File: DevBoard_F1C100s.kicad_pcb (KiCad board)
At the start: 2 copper layers, 192.8 x 140.2 mm, 51 parts, among them J101 USB_C_Receptacle_USB2.0_16P, J102 Conn_01x22, J103 Conn_01x11, J104 SD_Card, J105 UART0, J106 Conn_01x10, J108 Conn_01x05, J109 Conn_01x02, SW101 SW0, SW102 SW1, SW103 SW2, SW104 SW3, SW105 RESET, U101 AMS1117, U102 AMS1117-3.3, U103 TPS562201DDCT, U104 W25Q16JVSS, U105 F1C100s, Y101 24Mhz

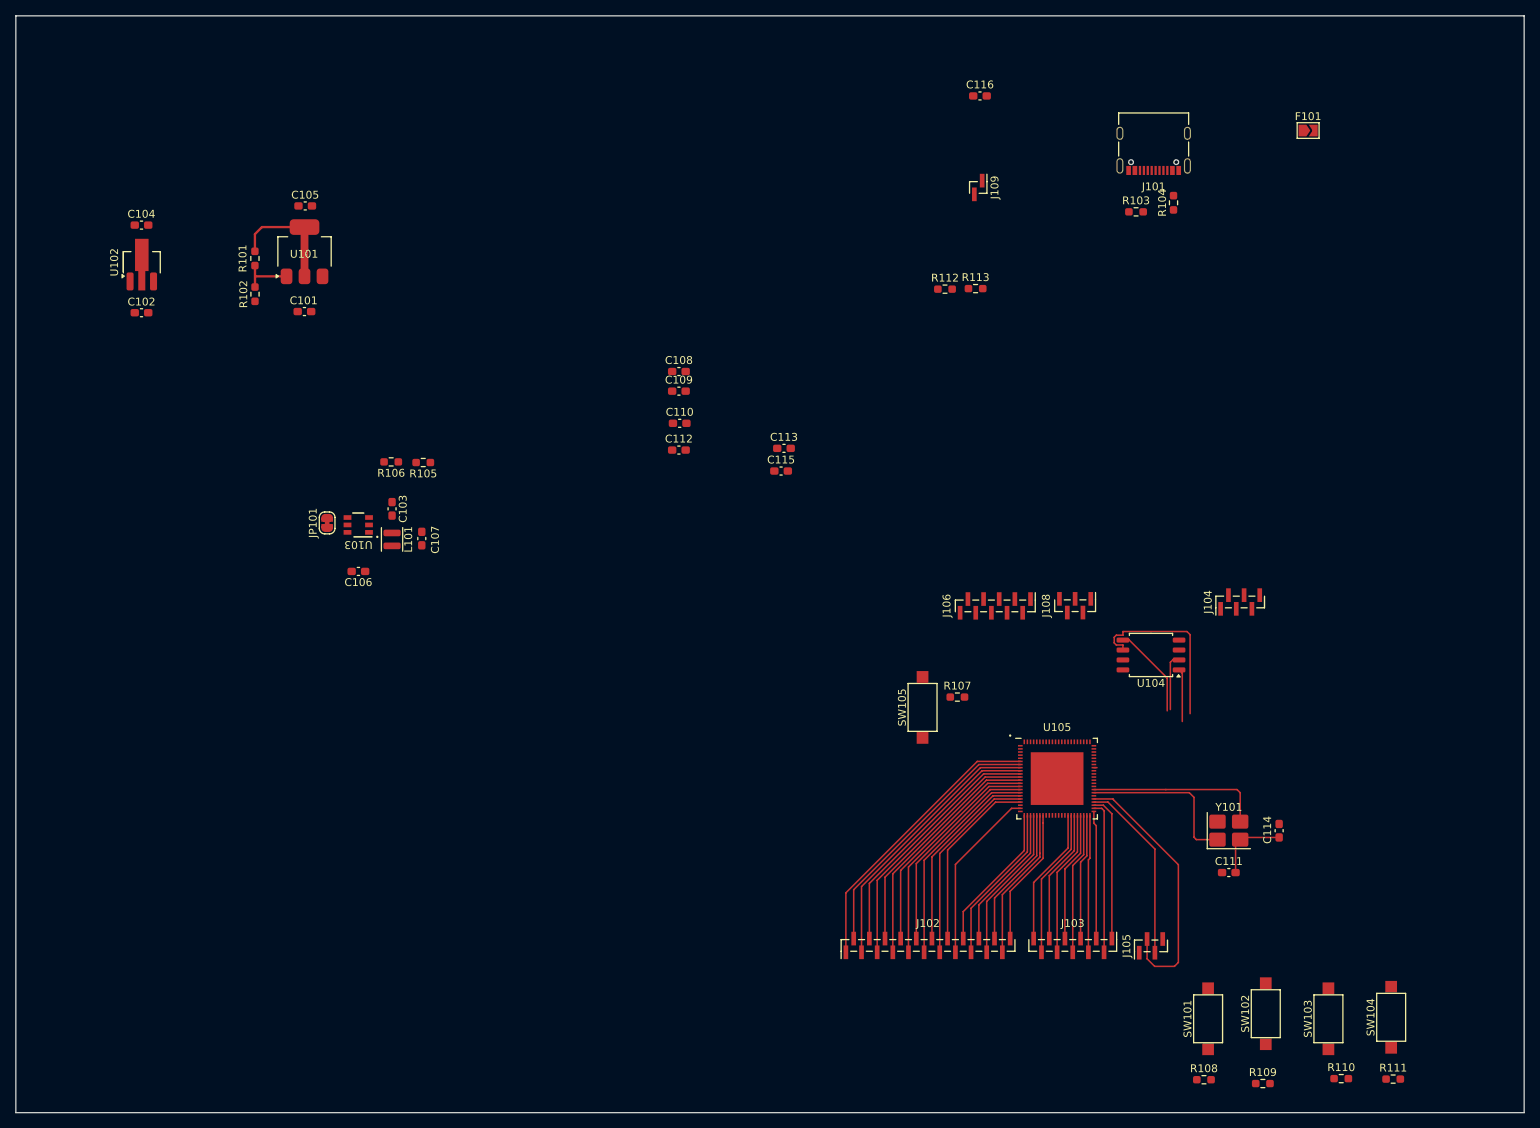
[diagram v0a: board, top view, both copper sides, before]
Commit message: Layout: Almost complete
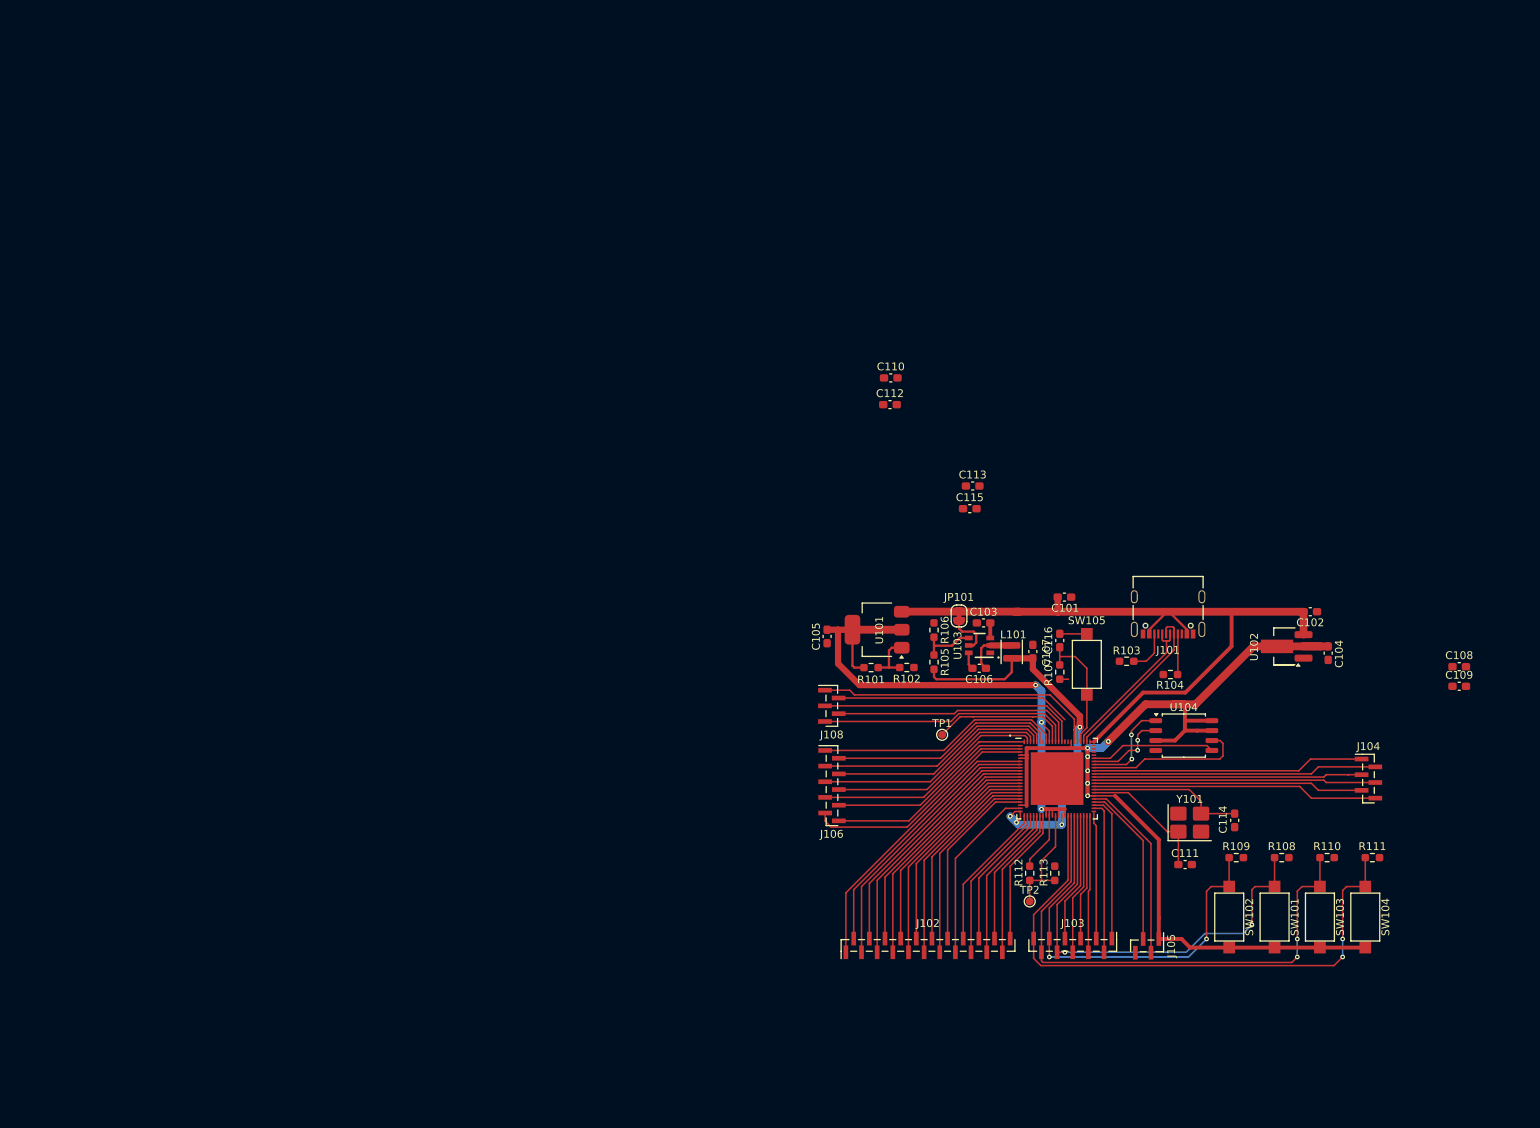
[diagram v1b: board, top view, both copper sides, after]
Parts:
- removed F101: 5V 2A, Jumper:SolderJumper-2_P1.3mm_Open_TrianglePad1.0x1.5mm
- removed J109: Conn_01x02, Connector_PinHeader_1.00mm:PinHeader_1x02_P1.00mm_Vertical_SMD_Pin1Left
- added TP1: TestPoint, TestPoint:TestPoint_Pad_D1.0mm, F.Cu at (140.3, 116.9)
- added TP2: TestPoint, TestPoint:TestPoint_Pad_D1.0mm, F.Cu at (151.5, 138.2)
- moved C104 161.3 mm to (189.7, 106.5), turned to -90 degrees
- moved C102 154.2 mm to (187.4, 101.2), turned to 0 degrees
- moved U102 154.1 mm to (184.1, 105.6), turned to 180 degrees
- moved C108 106.6 mm to (206.4, 108.2)
- moved C109 106.6 mm to (206.4, 110.7)
- moved C101 103.8 mm to (155.9, 99.3), turned to 0 degrees
- moved R102 96.0 mm to (135.8, 108.3), turned to 0 degrees
- moved R101 94.5 mm to (131.2, 108.3), turned to 0 degrees
- moved U101 87.7 mm to (132.0, 103.5), turned to 180 degrees
- moved C105 86.5 mm to (125.6, 104.3), turned to -90 degrees
- moved JP101 81.6 mm to (142.5, 101.7)
- moved U103 80.9 mm to (145.1, 105.5)
- moved L101 80.5 mm to (149.2, 106.3)
- moved C106 80.3 mm to (145.0, 108.4)
- moved C107 79.4 mm to (151.9, 106.3)
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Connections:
- C101 pad 1: /PWR_F -> /VUSB
- C102 pad 1: /PWR_F -> /VUSB
- C103 pad 1: /PWR_F -> /VUSB
- J101 pad A4: /VBUS -> /VUSB
- J101 pad A9: /VBUS -> /VUSB
- J101 pad B4: /VBUS -> /VUSB
- J101 pad B9: /VBUS -> /VUSB
- JP101 pad 2: /PWR_F -> /VUSB
- U101 pad 3: /PWR_F -> /VUSB
- U102 pad 3: /PWR_F -> /VUSB
- U103 pad 3: /PWR_F -> /VUSB
- U105 pad 67: /PWR_F -> /VUSB
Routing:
- net /3V3: track 0.00 -> 137.3 mm, vias 0 -> 6
- net /VUSB: track 0.00 -> 94.0 mm
- net /2V6: track 15.2 -> 80.2 mm, vias 0 -> 3
- net /SW3: track 17.6 -> 75.9 mm, vias 0 -> 2
- net /1V1: track 0.00 -> 55.3 mm, vias 0 -> 4
- net /SW2: track 19.1 -> 68.6 mm, vias 0 -> 2
- net /SW0: track 18.6 -> 56.2 mm, vias 0 -> 2
- net /SDC0_D2: track 0.00 -> 36.6 mm
- net /SW1: track 17.1 -> 53.4 mm, vias 0 -> 2
- net /SDC0_D0: track 0.00 -> 36.3 mm
- net /TVOUT: track 0.00 -> 36.3 mm
- net /SDC0_CMD: track 0.00 -> 36.1 mm
- net /SDC0_D1: track 0.00 -> 34.8 mm
- net /SDC0_D3: track 0.00 -> 34.6 mm
- net /SDC0_CLK: track 0.00 -> 34.4 mm
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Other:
- board outline removed

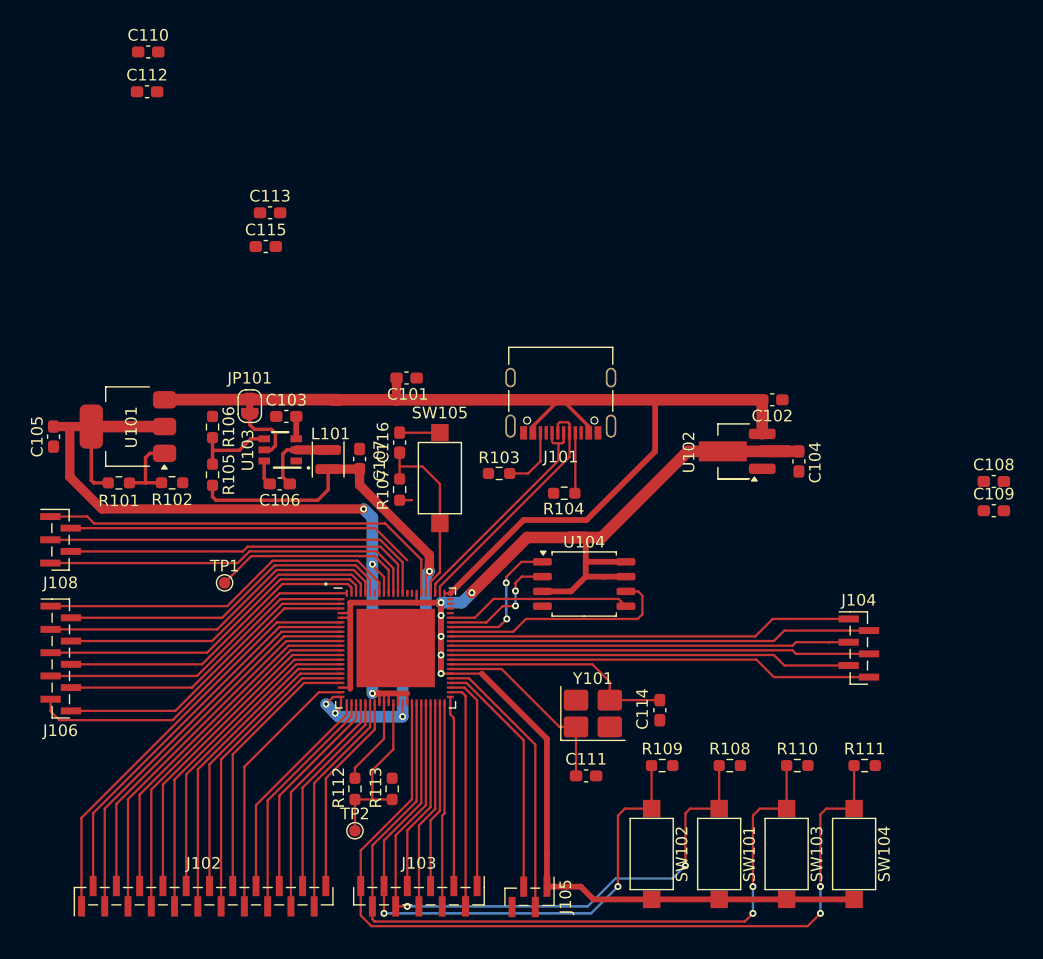
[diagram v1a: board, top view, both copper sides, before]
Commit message: Finish design
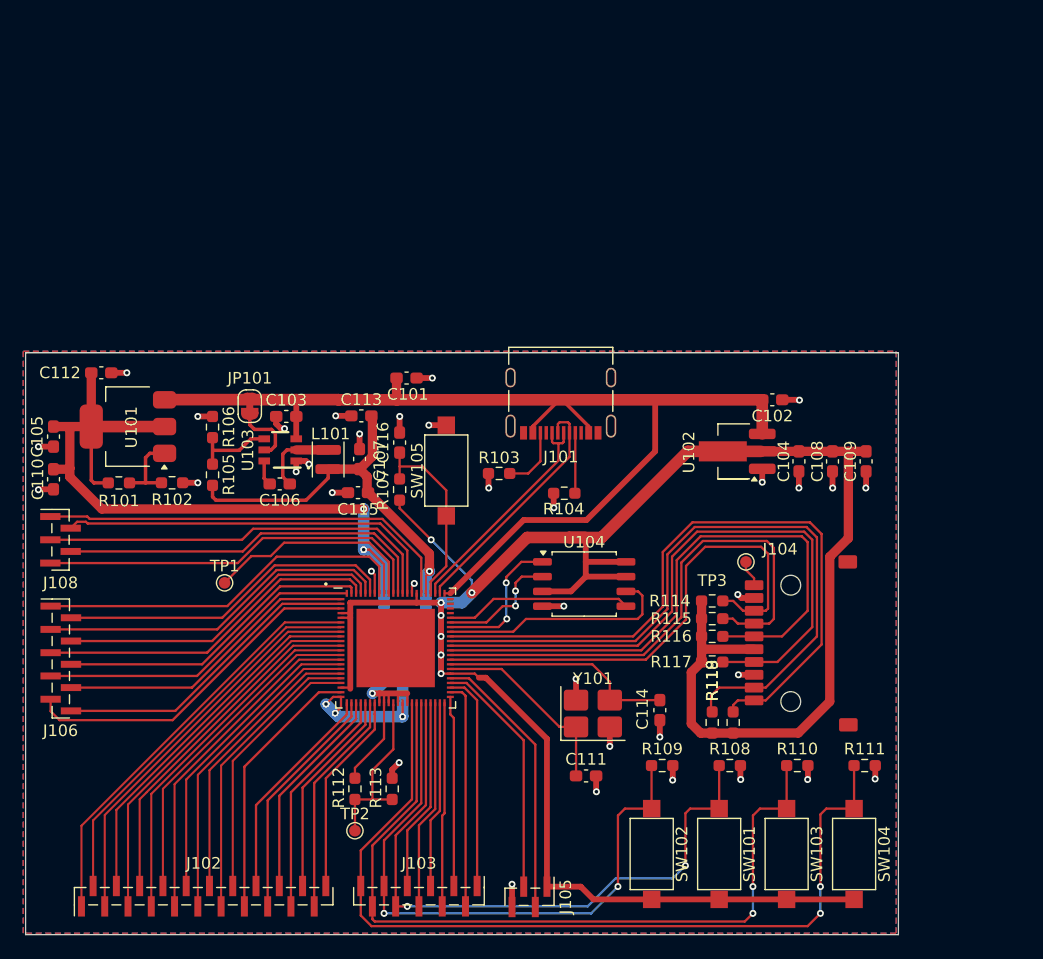
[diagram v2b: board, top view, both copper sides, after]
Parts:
- added R114: 10k, Resistor_SMD:R_0603_1608Metric_Pad0.98x0.95mm_HandSolder, F.Cu at (182.2, 118.5)
- added R115: 10k, Resistor_SMD:R_0603_1608Metric_Pad0.98x0.95mm_HandSolder, F.Cu at (182.2, 120.0)
- added R116: 10k, Resistor_SMD:R_0603_1608Metric_Pad0.98x0.95mm_HandSolder, F.Cu at (182.2, 121.5)
- added R117: 10k, Resistor_SMD:R_0603_1608Metric_Pad0.98x0.95mm_HandSolder, F.Cu at (182.2, 123.7)
- added R118: 10k, Resistor_SMD:R_0603_1608Metric_Pad0.98x0.95mm_HandSolder, F.Cu at (182.2, 128.9)
- added R119: 10k, Resistor_SMD:R_0603_1608Metric_Pad0.98x0.95mm_HandSolder, F.Cu at (184.0, 128.9)
- added TP3: TestPoint, TestPoint:TestPoint_Pad_D1.0mm, F.Cu at (185.1, 115.1)
- J104: value SD_Card -> Micro_SD_Card_Det1; footprint Connector_PinHeader_1.00mm:PinHeader_1x06_P1.00mm_Vertical_SMD_Pin1Left -> sd_card:sd_card_10p
- moved C110 37.6 mm to (125.6, 108.0), turned to -90 degrees
- moved C112 24.5 mm to (129.7, 98.8)
- moved C115 22.6 mm to (151.8, 109.2), turned to 180 degrees
- moved C113 19.1 mm to (152.1, 102.5), turned to 180 degrees
- moved C108 14.0 mm to (192.5, 106.5), turned to -90 degrees
- moved C109 11.8 mm to (195.4, 106.5), turned to -90 degrees
- moved J104 10.9 mm to (186.3, 129.4)
- moved SW105 0.85 mm to (159.3, 107.2)
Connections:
- J104 pad 1: /SDC0_D1 -> /SDC0_D2
- J104 pad 2: /SDC0_D0 -> /SDC0_D3
- J104 pad 3: /SDC0_CLK -> /SDC0_CMD
- J104 pad 4: /SDC0_CMD -> /3V3
- J104 pad 5: /SDC0_D3 -> /SDC0_CLK
- J104 pad 6: /SDC0_D2 -> GND
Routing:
- net /3V3: track 137.3 -> 200.8 mm, vias 6 -> 7
- net GND: track 3.47 -> 50.2 mm, vias 0 -> 36
- net /SDC0_D1: track 34.8 -> 59.0 mm
- net /SDC0_D0: track 36.3 -> 59.7 mm
- net /SDC0_CLK: track 34.4 -> 54.6 mm
- net /SDC0_CMD: track 36.1 -> 51.8 mm
- net /SDC0_D3: track 34.6 -> 45.7 mm
- net /2V6: track 80.2 -> 89.2 mm
- net /SDC0_D2: track 36.6 -> 43.3 mm
- net /1V1: track 55.3 -> 59.7 mm
- net /TV_VRN: track 30.2 -> 33.9 mm
- net Net-(J104-DET): track 0.00 -> 2.29 mm
- net /TVIN0: track 32.7 -> 34.0 mm
- net /LRADC0: track 17.6 -> 18.9 mm
- net /TVIN1: track 31.4 -> 32.7 mm
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- added copper zone on B.Cu, net GND
- added copper zone on F.Cu, net GND
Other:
- board outline added: 75 x 50 mm
